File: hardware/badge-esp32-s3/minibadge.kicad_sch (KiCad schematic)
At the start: 10 parts, among them J10 Conn_01x02_Socket, J3 Conn_01x02_Socket, J4 Conn_01x02_Socket, J5 Conn_01x02_Socket, J6 Conn_01x04_Socket, J7 Conn_01x02_Socket, J8 Conn_01x04_Socket, J9 Conn_01x02_Socket

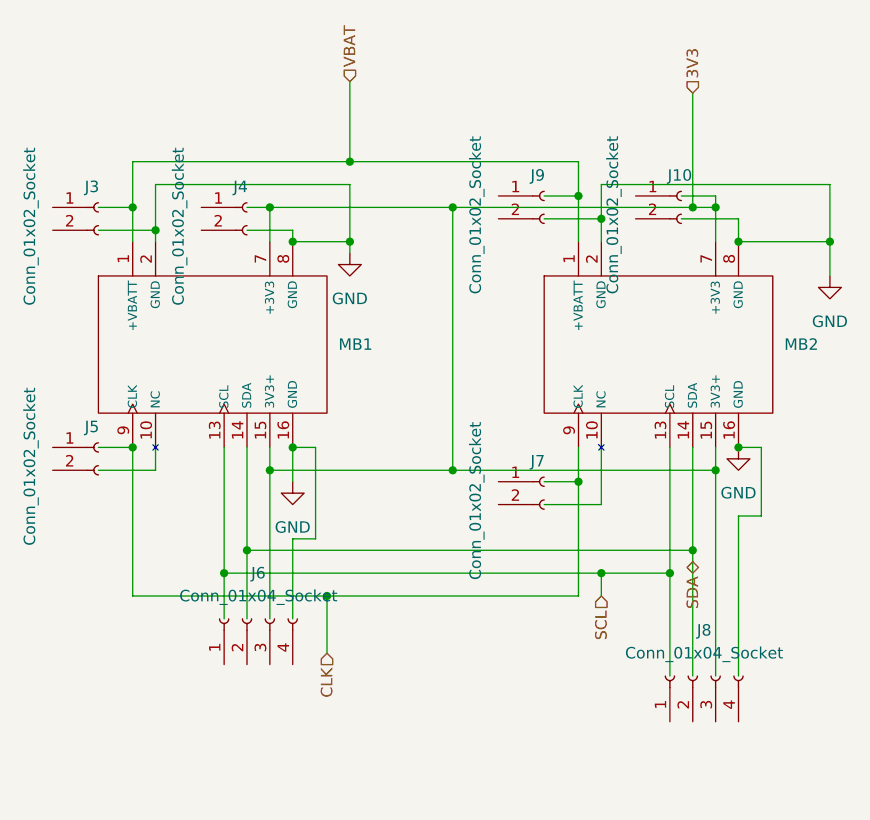
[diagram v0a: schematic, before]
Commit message: minibadge_fix_update
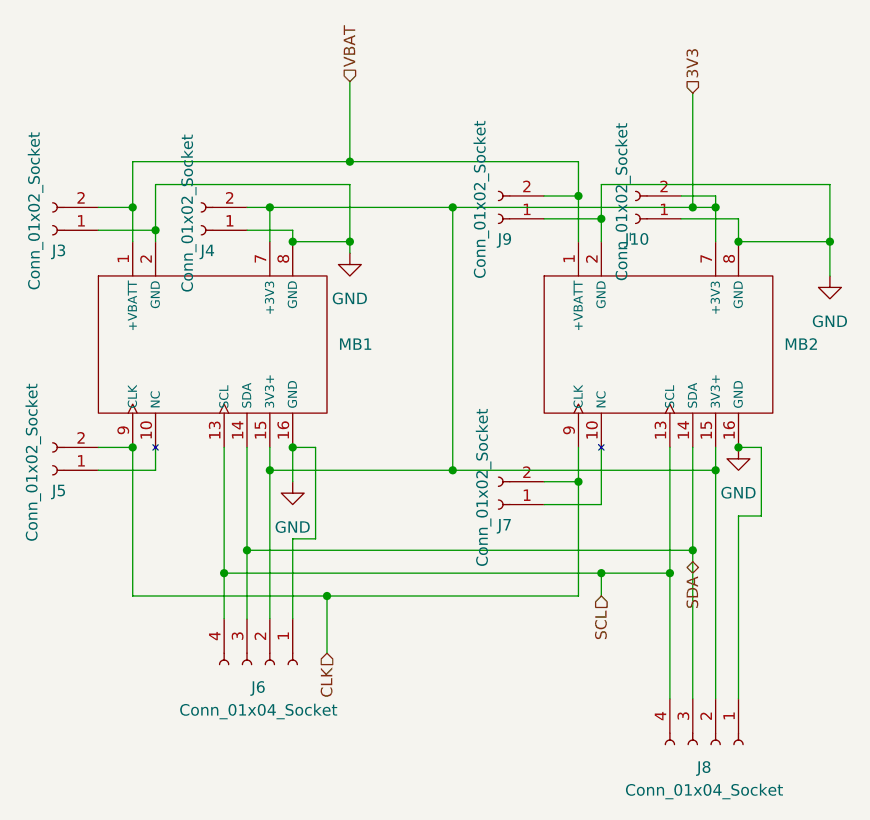
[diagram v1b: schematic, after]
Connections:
- net 3V3: now also J10.2 (Pin_2), J4.2 (Pin_2), J6.2 (Pin_2), J8.2 (Pin_2)
- net CLK: now also J5.2 (Pin_2), J7.2 (Pin_2)
- net GND: now also J10.1 (Pin_1), J3.1 (Pin_1), J4.1 (Pin_1), J6.1 (Pin_1), J8.1 (Pin_1), J9.1 (Pin_1)
- net SCL: now also J6.4 (Pin_4), J8.4 (Pin_4)
- net SDA: now also J6.3 (Pin_3), J8.3 (Pin_3)
- net VBAT: now also J3.2 (Pin_2), J9.2 (Pin_2)
- net at J5.1 (Pin_1): now also MB1.10 (NC)
- net at J7.1 (Pin_1): now also MB2.10 (NC)
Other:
- moved on the sheet: J10, J3, J4, J5, J6, J7, J8, J9
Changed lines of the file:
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@@
+	(wire
+		(pts
+			(xy 154.94 100.33) (xy 154.94 114.3)
+		)
+		(stroke
+			(width 0)
+			(type default)
+		)
+	)
 	(wire
 		(pts
@@
 	(wire
 		(pts
+			(xy 157.48 97.79) (xy 157.48 114.3)
+		)
+		(stroke
+			(width 0)
+			(type default)
+		)
+	)
+	(wire
+		(pts
 			(xy 160.02 59.69) (xy 160.02 63.5)
 		)
@@
 	(wire
 		(pts
+			(xy 162.56 93.98) (xy 162.56 114.3)
+		)
+		(stroke
+			(width 0)
+			(type default)
+		)
+	)
+	(wire
+		(pts
 			(xy 113.03 105.41) (xy 113.03 96.52)
 		)
@@
 	(wire
 		(pts
-			(xy 154.94 100.33) (xy 154.94 111.76)
-		)
-		(stroke
-			(width 0)
-			(type default)
-		)
-	)
-	(wire
-		(pts
 			(xy 147.32 57.15) (xy 172.72 57.15)
 		)
@@
 	(wire
 		(pts
-			(xy 157.48 97.79) (xy 157.48 111.76)
-		)
-		(stroke
-			(width 0)
-			(type default)
-		)
-	)
-	(wire
-		(pts
 			(xy 165.1 93.98) (xy 165.1 86.36)
 		)
@@
 	(wire
 		(pts
-			(xy 162.56 93.98) (xy 162.56 111.76)
+			(xy 160.02 88.9) (xy 160.02 114.3)
 		)
 		(stroke
@@
 		(pts
 			(xy 105.41 100.33) (xy 147.32 100.33)
-		)
-		(stroke
-			(width 0)
-			(type default)
-		)
-	)
-	(wire
-		(pts
-			(xy 160.02 88.9) (xy 160.02 111.76)
 		)
 		(stroke
@@
 	(symbol
 		(lib_id "Connector:Conn_01x02_Socket")
-		(at 91.44 86.36 0)
+		(at 86.36 88.9 180)
 		(unit 1)
 		(exclude_from_sim no)
@@
 		(dnp no)
 		(property "Reference" "J5"
-			(at 89.916 84.074 0)
+			(at 87.884 91.186 0)
 			(effects
 				(font
@@
 		)
 		(property "Value" "Conn_01x02_Socket"
-			(at 83.82 97.282 90)
+			(at 84.074 79.248 90)
 			(effects
 				(font
@@
 		)
 		(property "Footprint" "Connector_PinHeader_2.54mm:PinHeader_1x02_P2.54mm_Vertical"
-			(at 91.44 86.36 0)
+			(at 86.36 88.9 0)
 			(effects
 				(font
@@
 		)
 		(property "Datasheet" "~"
-			(at 91.44 86.36 0)
+			(at 86.36 88.9 0)
 			(effects
 				(font
@@
 		)
 		(property "Description" "Generic connector, single row, 01x02, script generated"
-			(at 91.44 86.36 0)
+			(at 86.36 88.9 0)
 			(effects
 				(font
@@
 	(symbol
 		(lib_id "Connector:Conn_01x02_Socket")
-		(at 140.97 90.17 0)
+		(at 135.89 92.71 180)
 		(unit 1)
 		(exclude_from_sim no)
@@
 		(dnp no)
 		(property "Reference" "J7"
-			(at 139.446 87.884 0)
+			(at 137.414 94.996 0)
 			(effects
 				(font
@@
 		)
 		(property "Value" "Conn_01x02_Socket"
-			(at 133.35 101.092 90)
+			(at 134.112 82.042 90)
 			(effects
 				(font
@@
 		)
 		(property "Footprint" "Connector_PinHeader_2.54mm:PinHeader_1x02_P2.54mm_Vertical"
-			(at 140.97 90.17 0)
+			(at 135.89 92.71 0)
 			(effects
 				(font
@@
 		)
 		(property "Datasheet" "~"
-			(at 140.97 90.17 0)
+			(at 135.89 92.71 0)
 			(effects
 				(font
@@
 		)
 		(property "Description" "Generic connector, single row, 01x02, script generated"
-			(at 140.97 90.17 0)
+			(at 135.89 92.71 0)
 			(effects
 				(font
@@
 	(symbol
 		(lib_id "Connector:Conn_01x02_Socket")
-		(at 91.44 59.69 0)
+		(at 86.36 62.23 180)
 		(unit 1)
 		(exclude_from_sim no)
@@
 		(dnp no)
 		(property "Reference" "J3"
-			(at 89.916 57.404 0)
+			(at 87.884 64.516 0)
 			(effects
 				(font
@@
 		)
 		(property "Value" "Conn_01x02_Socket"
-			(at 83.82 70.612 90)
+			(at 84.328 51.308 90)
 			(effects
 				(font
@@
 		)
 		(property "Footprint" "Connector_PinHeader_2.54mm:PinHeader_1x02_P2.54mm_Vertical"
-			(at 91.44 59.69 0)
+			(at 86.36 62.23 0)
 			(effects
 				(font
@@
 		)
 		(property "Datasheet" "~"
-			(at 91.44 59.69 0)
+			(at 86.36 62.23 0)
 			(effects
 				(font
@@
 		)
 		(property "Description" "Generic connector, single row, 01x02, script generated"
-			(at 91.44 59.69 0)
+			(at 86.36 62.23 0)
 			(effects
 				(font
@@
 		)
 		(instances
-			(project ""
+			(project "badge-esp32-s3"
 				(path "/e2af9a6c-dbe9-4de2-9ba6-ea213a7300ec/18b0dd1f-1411-4aae-8334-5d13e6c2c6f9"
 					(reference "J3")
@@
 	(symbol
 		(lib_id "Connector:Conn_01x02_Socket")
-		(at 156.21 58.42 0)
+		(at 151.13 60.96 180)
 		(unit 1)
 		(exclude_from_sim no)
@@
 		(dnp no)
 		(property "Reference" "J10"
-			(at 154.686 56.134 0)
+			(at 152.654 63.246 0)
 			(effects
 				(font
@@
 		)
 		(property "Value" "Conn_01x02_Socket"
-			(at 148.59 69.342 90)
+			(at 149.606 50.292 90)
 			(effects
 				(font
@@
 		)
 		(property "Footprint" "Connector_PinHeader_2.54mm:PinHeader_1x02_P2.54mm_Vertical"
-			(at 156.21 58.42 0)
+			(at 151.13 60.96 0)
 			(effects
 				(font
@@
 		)
 		(property "Datasheet" "~"
-			(at 156.21 58.42 0)
+			(at 151.13 60.96 0)
 			(effects
 				(font
@@
 		)
 		(property "Description" "Generic connector, single row, 01x02, script generated"
-			(at 156.21 58.42 0)
+			(at 151.13 60.96 0)
 			(effects
 				(font
@@
 	(symbol
 		(lib_id "Connector:Conn_01x04_Socket")
-		(at 107.95 105.41 90)
+		(at 110.49 110.49 270)
 		(unit 1)
 		(exclude_from_sim no)
@@
 		(fields_autoplaced yes)
 		(property "Reference" "J6"
-			(at 109.22 100.33 90)
+			(at 109.22 113.03 90)
 			(effects
 				(font
@@
 		)
 		(property "Value" "Conn_01x04_Socket"
-			(at 109.22 102.87 90)
+			(at 109.22 115.57 90)
 			(effects
 				(font
@@
 		)
 		(property "Footprint" "Connector_PinHeader_2.54mm:PinHeader_1x04_P2.54mm_Vertical"
-			(at 107.95 105.41 0)
+			(at 110.49 110.49 0)
 			(effects
 				(font
@@
 		)
 		(property "Datasheet" "~"
-			(at 107.95 105.41 0)
+			(at 110.49 110.49 0)
 			(effects
 				(font
@@
 		)
 		(property "Description" "Generic connector, single row, 01x04, script generated"
-			(at 107.95 105.41 0)
+			(at 110.49 110.49 0)
 			(effects
 				(font
@@
 		)
 		(instances
-			(project ""
+			(project "badge-esp32-s3"
 				(path "/e2af9a6c-dbe9-4de2-9ba6-ea213a7300ec/18b0dd1f-1411-4aae-8334-5d13e6c2c6f9"
 					(reference "J6")
@@
 	(symbol
 		(lib_id "Connector:Conn_01x02_Socket")
-		(at 107.95 59.69 0)
+		(at 102.87 62.23 180)
 		(unit 1)
 		(exclude_from_sim no)
@@
 		(dnp no)
 		(property "Reference" "J4"
-			(at 106.426 57.404 0)
+			(at 104.394 64.516 0)
 			(effects
 				(font
@@
 		)
 		(property "Value" "Conn_01x02_Socket"
-			(at 100.33 70.612 90)
+			(at 101.346 51.562 90)
 			(effects
 				(font
@@
 		)
 		(property "Footprint" "Connector_PinHeader_2.54mm:PinHeader_1x02_P2.54mm_Vertical"
-			(at 107.95 59.69 0)
+			(at 102.87 62.23 0)
 			(effects
 				(font
@@
 		)
 		(property "Datasheet" "~"
-			(at 107.95 59.69 0)
+			(at 102.87 62.23 0)
 			(effects
 				(font
@@
 		)
 		(property "Description" "Generic connector, single row, 01x02, script generated"
-			(at 107.95 59.69 0)
+			(at 102.87 62.23 0)
 			(effects
 				(font
@@
 	(symbol
 		(lib_id "Connector:Conn_01x02_Socket")
-		(at 140.97 58.42 0)
+		(at 135.89 60.96 180)
 		(unit 1)
 		(exclude_from_sim no)
@@
 		(dnp no)
 		(property "Reference" "J9"
-			(at 139.446 56.134 0)
+			(at 137.414 63.246 0)
 			(effects
 				(font
@@
 		)
 		(property "Value" "Conn_01x02_Socket"
-			(at 133.35 69.342 90)
+			(at 133.858 50.038 90)
 			(effects
 				(font
@@
 		)
 		(property "Footprint" "Connector_PinHeader_2.54mm:PinHeader_1x02_P2.54mm_Vertical"
-			(at 140.97 58.42 0)
+			(at 135.89 60.96 0)
 			(effects
 				(font
@@
 		)
 		(property "Datasheet" "~"
-			(at 140.97 58.42 0)
+			(at 135.89 60.96 0)
 			(effects
 				(font
@@
 		)
 		(property "Description" "Generic connector, single row, 01x02, script generated"
-			(at 140.97 58.42 0)
+			(at 135.89 60.96 0)
 			(effects
 				(font
@@
 	(symbol
 		(lib_id "Connector:Conn_01x04_Socket")
-		(at 157.48 111.76 90)
+		(at 160.02 119.38 270)
 		(unit 1)
 		(exclude_from_sim no)
@@
 		(fields_autoplaced yes)
 		(property "Reference" "J8"
-			(at 158.75 106.68 90)
+			(at 158.75 121.92 90)
 			(effects
 				(font
@@
 		)
 		(property "Value" "Conn_01x04_Socket"
-			(at 158.75 109.22 90)
+			(at 158.75 124.46 90)
 			(effects
 				(font
@@
 		)
 		(property "Footprint" "Connector_PinHeader_2.54mm:PinHeader_1x04_P2.54mm_Vertical"
-			(at 157.48 111.76 0)
+			(at 160.02 119.38 0)
 			(effects
 				(font
@@
 		)
 		(property "Datasheet" "~"
-			(at 157.48 111.76 0)
+			(at 160.02 119.38 0)
 			(effects
 				(font
@@
 		)
 		(property "Description" "Generic connector, single row, 01x04, script generated"
-			(at 157.48 111.76 0)
-			(effects
-				(font
+			(at 160.02 119.38 0)
+			(effects
+				(font

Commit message: Minibadge_final??
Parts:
- J10, J3, J4, J5, J7, J9: footprint Connector_PinHeader_2.54mm:PinHeader_1x02_P2.54mm_Vertical -> Connector_PinSocket_2.54mm:PinSocket_1x02_P2.54mm_Vertical
- J6, J8: footprint Connector_PinHeader_2.54mm:PinHeader_1x04_P2.54mm_Vertical -> Connector_PinSocket_2.54mm:PinSocket_1x04_P2.54mm_Vertical
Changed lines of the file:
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@@
 			)
 		)
-		(property "Footprint" "Connector_PinHeader_2.54mm:PinHeader_1x02_P2.54mm_Vertical"
+		(property "Footprint" "Connector_PinSocket_2.54mm:PinSocket_1x02_P2.54mm_Vertical"
 			(at 86.36 88.9 0)
 			(effects
@@
 			)
 		)
-		(property "Footprint" "Connector_PinHeader_2.54mm:PinHeader_1x02_P2.54mm_Vertical"
+		(property "Footprint" "Connector_PinSocket_2.54mm:PinSocket_1x02_P2.54mm_Vertical"
 			(at 135.89 92.71 0)
 			(effects
@@
 			)
 		)
-		(property "Footprint" "Connector_PinHeader_2.54mm:PinHeader_1x02_P2.54mm_Vertical"
+		(property "Footprint" "Connector_PinSocket_2.54mm:PinSocket_1x02_P2.54mm_Vertical"
 			(at 86.36 62.23 0)
 			(effects
@@
 			)
 		)
-		(property "Footprint" "Connector_PinHeader_2.54mm:PinHeader_1x02_P2.54mm_Vertical"
+		(property "Footprint" "Connector_PinSocket_2.54mm:PinSocket_1x02_P2.54mm_Vertical"
 			(at 151.13 60.96 0)
 			(effects
@@
 			)
 		)
-		(property "Footprint" "Connector_PinHeader_2.54mm:PinHeader_1x04_P2.54mm_Vertical"
+		(property "Footprint" "Connector_PinSocket_2.54mm:PinSocket_1x04_P2.54mm_Vertical"
 			(at 110.49 110.49 0)
 			(effects
@@
 			)
 		)
-		(property "Footprint" "Connector_PinHeader_2.54mm:PinHeader_1x02_P2.54mm_Vertical"
+		(property "Footprint" "Connector_PinSocket_2.54mm:PinSocket_1x02_P2.54mm_Vertical"
 			(at 102.87 62.23 0)
 			(effects
@@
 			)
 		)
-		(property "Footprint" "Connector_PinHeader_2.54mm:PinHeader_1x02_P2.54mm_Vertical"
+		(property "Footprint" "Connector_PinSocket_2.54mm:PinSocket_1x02_P2.54mm_Vertical"
 			(at 135.89 60.96 0)
 			(effects
@@
 			)
 		)
-		(property "Footprint" "Connector_PinHeader_2.54mm:PinHeader_1x04_P2.54mm_Vertical"
+		(property "Footprint" "Connector_PinSocket_2.54mm:PinSocket_1x04_P2.54mm_Vertical"
 			(at 160.02 119.38 0)
 			(effects
